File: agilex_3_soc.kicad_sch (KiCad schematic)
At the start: 18 parts, among them J1 Conn_01x14, J2 Conn_02x03_Odd_Even, J3 Conn_02x19_Odd_Even, J4 Conn_01x03, J5 Conn_01x03, J6 Micro_SD_Card, J7 8P8C_LED_Shielded, U2 ADS7886xxDBV, U3 CD4051B, U5 IS43LQ32256A-062BLI, Y1 ASDMB-25MHz

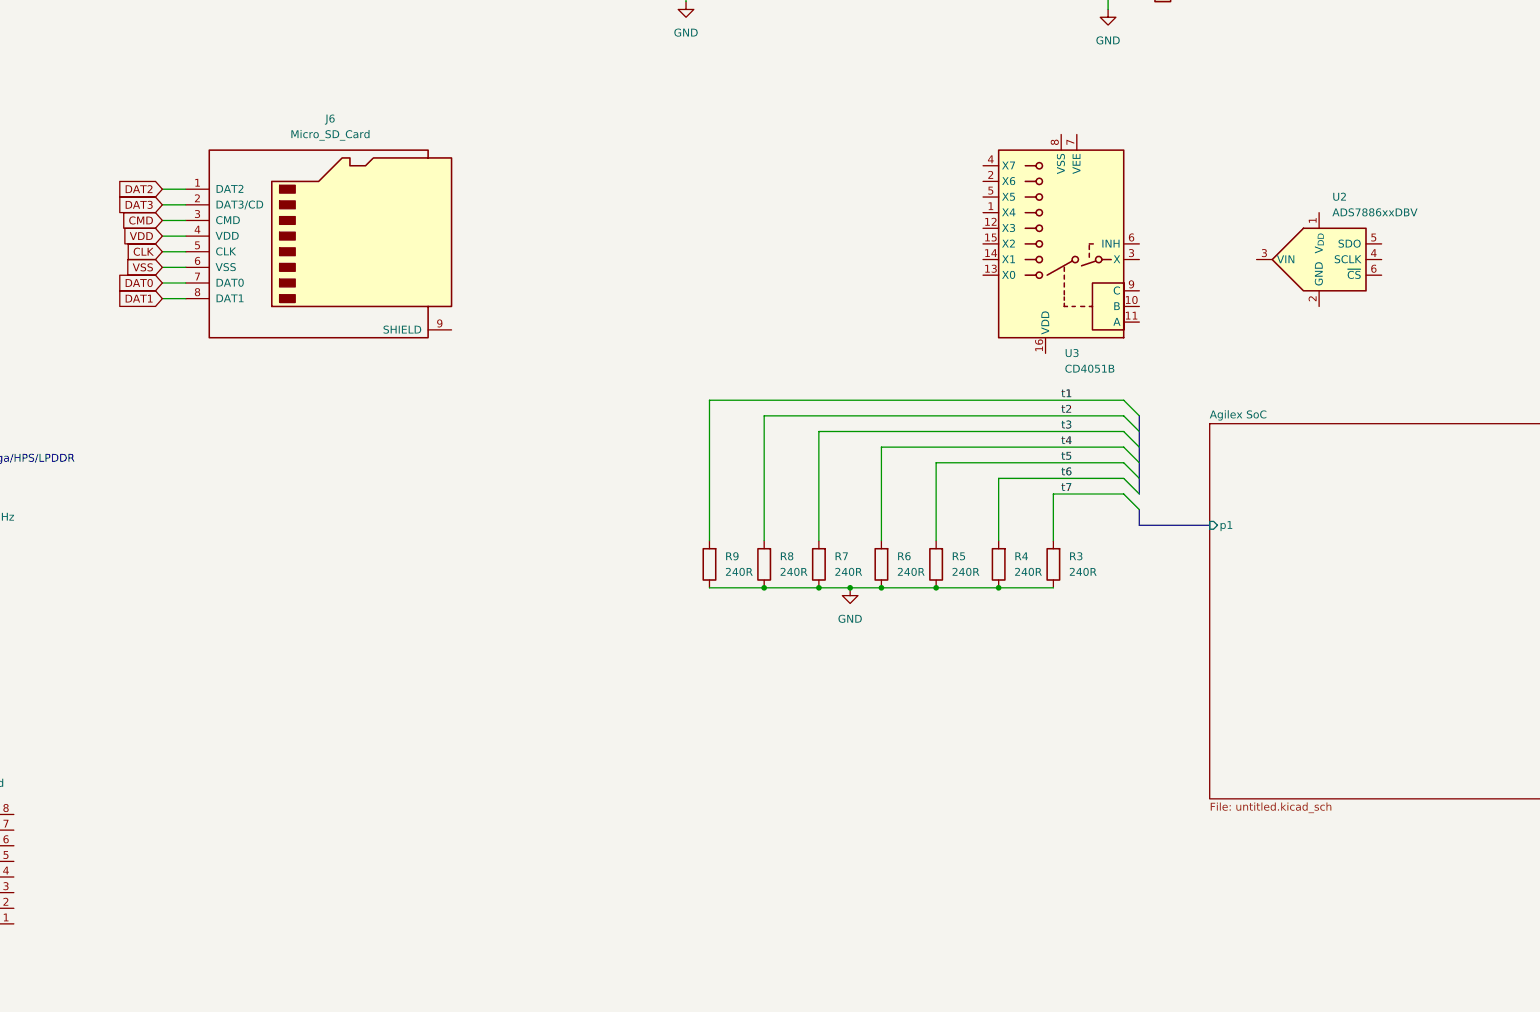
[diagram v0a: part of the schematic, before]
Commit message: sketch io routing between connector and agilex
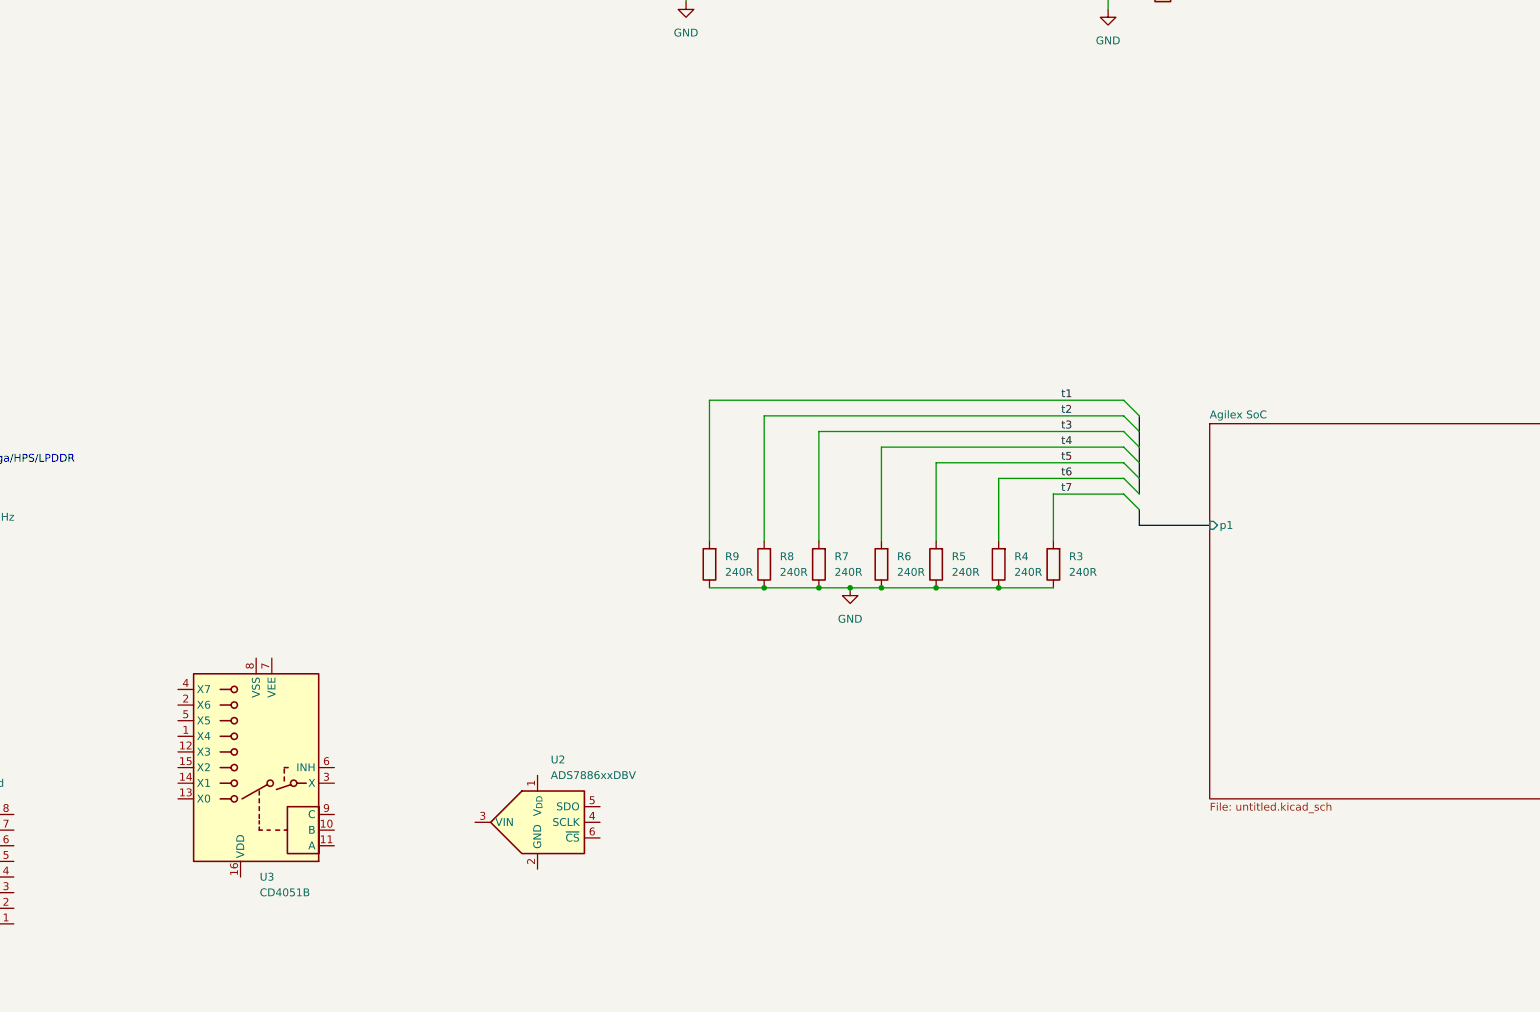
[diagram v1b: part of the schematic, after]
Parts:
- removed J6: Micro_SD_Card, Connector_Card:microSD_HC_Hirose_DM3AT-SF-PEJM5, symbol Connector:Micro_SD_Card
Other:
- moved on the sheet: U2, U3
